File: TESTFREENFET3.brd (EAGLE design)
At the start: 53.3 x 53.3 mm, 21 parts, among them J1 Digital_0_7, J2 Analog, J3 Digital_8_13

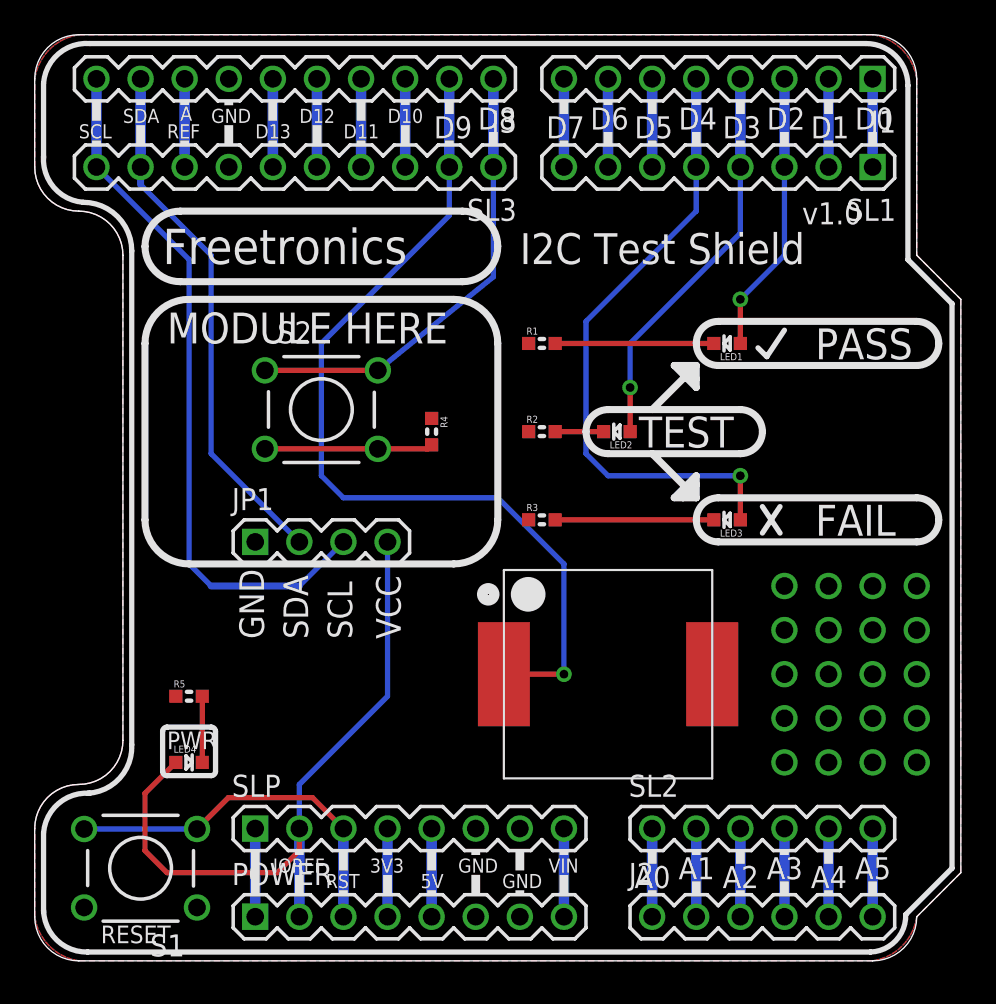
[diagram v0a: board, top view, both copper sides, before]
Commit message: Created TESTFREENFET3 project for release v1.0
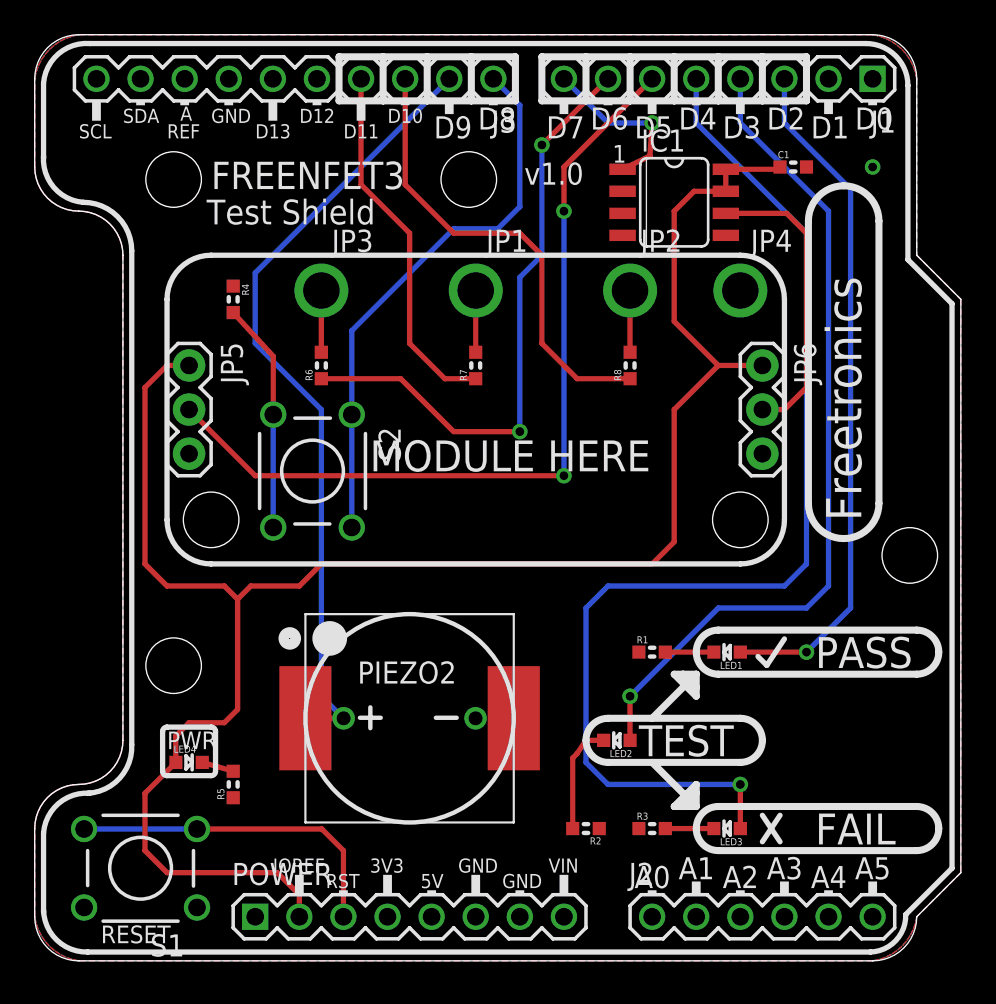
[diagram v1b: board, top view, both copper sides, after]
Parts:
- removed SL1: Digital_0_7, freetronics:1X08
- removed SL2: Analog, freetronics:1X06
- removed SL3: Digital_8_13, freetronics-original:1X10
- removed SLP: Power, freetronics:1X08
- added C1: 1uF 0603, freetronics-master-v1:0603
- added IC1: WS2811-SOP8, freetronics-jon:SO08-SKINNYPADS
- added JP2: DRAIN3, freetronics-jon:1X01_2_1_MM
- added JP3: DRAIN1, freetronics-jon:1X01_2_1_MM
- added JP4: SOURCE, freetronics-jon:1X01_2_1_MM
- added JP5: IN, freetronics-jon:1X03
- added JP6: OUT, freetronics-jon:1X03
- added PIEZO2: PIEZOPOLARISED, freetronics-jon:PIEZO12MMWIDEPOLARISED
- added R6, R7, R8: 1K, freetronics-jon:0603
- JP1: value MODULE -> DRAIN2; device freetronics-master-v1.1:1X04 -> freetronics-jon:1X01_2_1_MM
- R1, R2, R3: value 560R 0603 -> 560R
- R4: value 1K 0603 -> 1K
- R5: value 1K5 0603 -> 1K5
- moved R2 23.0 mm to (31.8, 7.62), turned to 180 degrees
- moved JP1 19.3 mm to (25.4, 38.6)
- moved R1 18.9 mm to (35.6, 17.8)
- moved R3 18.9 mm to (35.6, 7.62)
- moved LED1 17.8 mm to (39.9, 17.8)
- moved LED2 17.8 mm to (33.5, 12.7)
- moved LED3 17.8 mm to (39.9, 7.62)
- moved R4 13.7 mm to (11.4, 38.1)
- moved PIEZO 11.7 mm to (21.6, 14.0)
- moved R5 5.68 mm to (11.4, 10.2), turned to 90 degrees
- moved S2 3.58 mm to (16.0, 28.2), turned to 270 degrees
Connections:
- new net DIN: IC1.6, JP6.2
- new net N$5: JP3.1, R6.2
- new net N$6: JP1.1, R7.2
- new net N$8: JP2.1, R8.2
- new net OUT2: IC1.2
- new net OUT3: IC1.3
- net 3V3: no longer SLP.4
- net 5V: no longer SLP.5
- net A0: no longer SL2.1
- net A1: no longer SL2.2
- net A2: no longer SL2.3
- net A3: no longer SL2.4
- net A4: no longer SL2.5
- net A5: no longer SL2.6
- net AREF: no longer SL3.8
- net D0_RX: no longer SL1.1
- net D10: now also R8.1; no longer SL3.3
- net D11_MOSI: now also R7.1; no longer SL3.4
- net D12_MISO: no longer SL3.5
- net D13_SCK: no longer SL3.6
- net D1_TX: no longer SL1.2
- net D2: no longer SL1.3
- net D3: no longer SL1.4
- net D4: no longer SL1.5
- net D5: now also JP5.2; no longer SL1.6
- net D6: now also R6.1; no longer SL1.7
- net D7: now also IC1.1; no longer SL1.8
- net D8: no longer SL3.1
- net D9: now also PIEZO2.1; no longer SL3.2
- net GND: now also C1.2, IC1.4, JP4.1, JP5.3, JP6.3, PIEZO2.2; no longer JP1.1, SL3.7, SLP.6, SLP.7
- net IOREF: now also C1.1, IC1.7, IC1.8, JP5.1, JP6.1; no longer JP1.4, SLP.2
- net NC: no longer SLP.1
- net RESET: no longer SLP.3
- net SCL: no longer JP1.3, SL3.10
- net SDA: no longer JP1.2, SL3.9
- net VIN: no longer SLP.8
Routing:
- net IOREF: track 40.7 -> 106.6 mm
- net D5: track 5.08 -> 48.1 mm, vias 0 -> 2
- net SCL: track 40.6 -> 0.00 mm
- net SDA: track 30.5 -> 0.00 mm
- net D6: track 5.08 -> 35.1 mm, vias 0 -> 2
- net D4: track 36.2 -> 65.2 mm
- net D3: track 23.0 -> 47.9 mm
- net D2: track 16.3 -> 39.5 mm
- net D10: track 5.08 -> 26.7 mm
- net DIN: track 0.00 -> 17.1 mm
- net D11_MOSI: track 5.08 -> 21.0 mm
- net N$3: track 9.14 -> 2.79 mm
- net N$1: track 9.14 -> 2.79 mm
- net D9: track 51.8 -> 45.8 mm, vias 1 -> 0
- net D8: track 26.5 -> 32.0 mm
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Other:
- board text added: "(c) 2017 Freetronics Pty Ltd"
- board text added: "1"
- board text added: "D2: GREEN (PASS) D3: YELLOW (BEGIN) D4: RED (FAIL) D5: TESTDATA D6: TESTSENSE1 D7: OUTPUTSENSE D8: DETECT D9: PIEZO D10: TESTSENSE2 D11: TESTSENSE3"
- board text added: "FREENFET3"
- board text added: "K"
- board text added: "Test Shield"
- board text added: "www.freetronics.com.au"
- board text removed: "(c) 2014 Freetronics Pty Ltd"
- board text removed: "D2: PASS D3: TEST D4: FAIL D8: nDETECT D9: PIEZO"
- board text removed: "I2C Test Shield"
- board text removed: "VCC"
- board text removed: "www.freetronics.com"
